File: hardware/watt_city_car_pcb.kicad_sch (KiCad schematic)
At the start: 0 parts

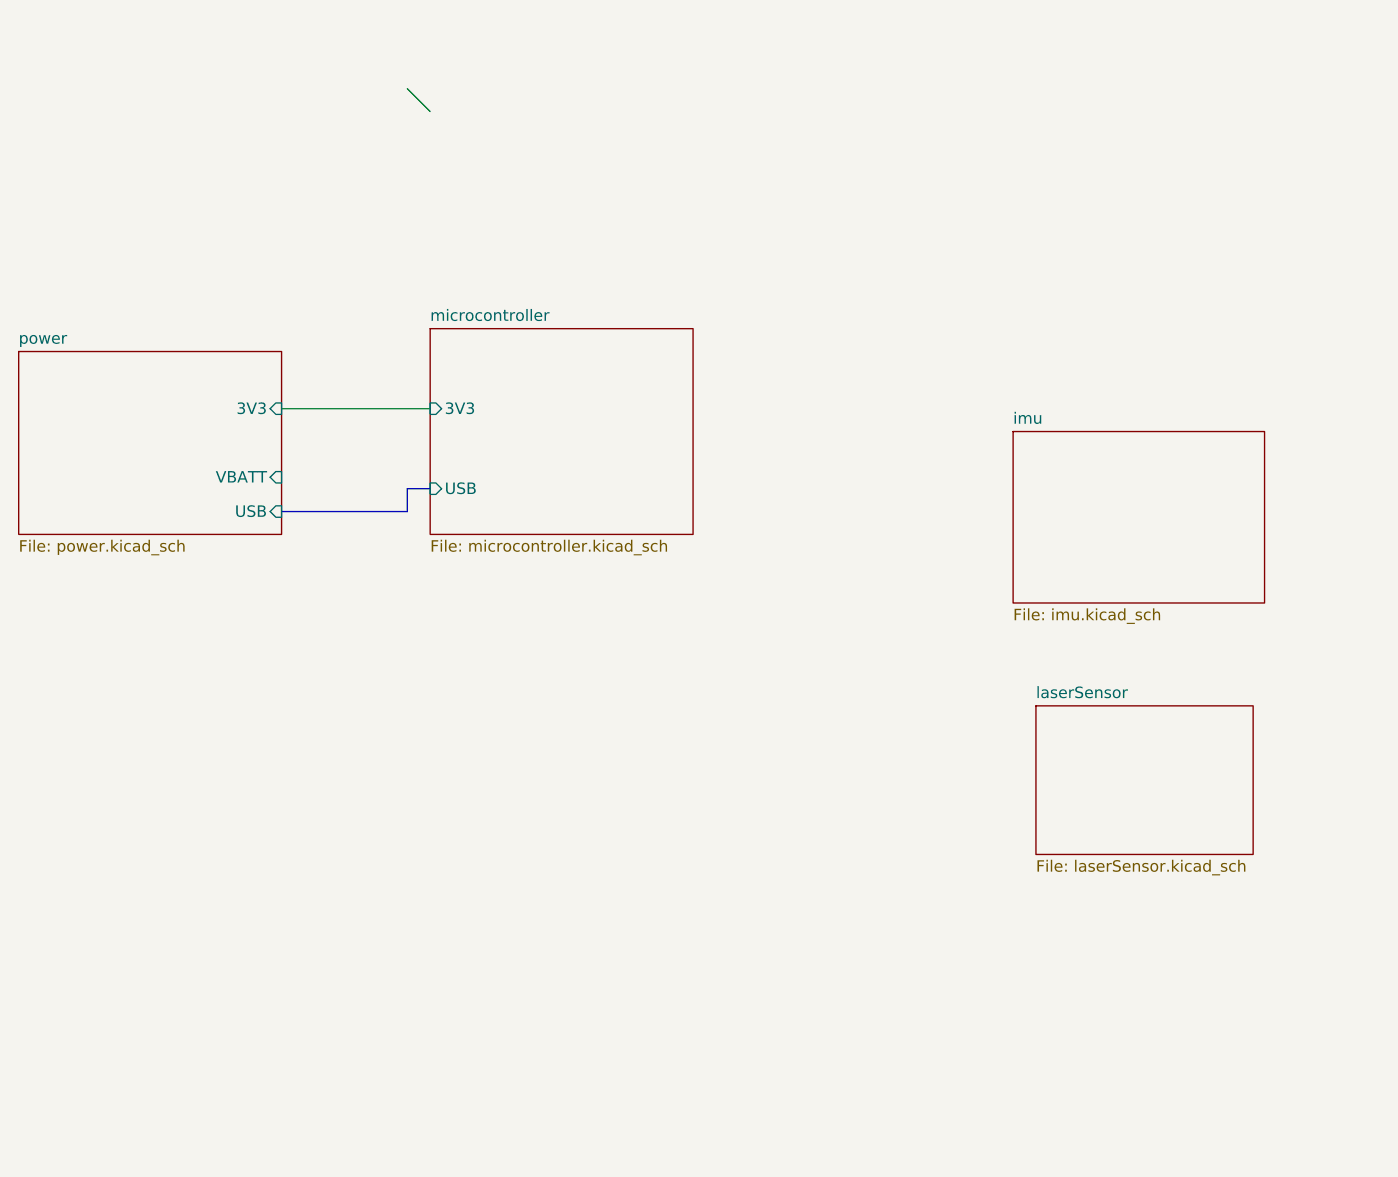
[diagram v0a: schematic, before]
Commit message: updated pcb
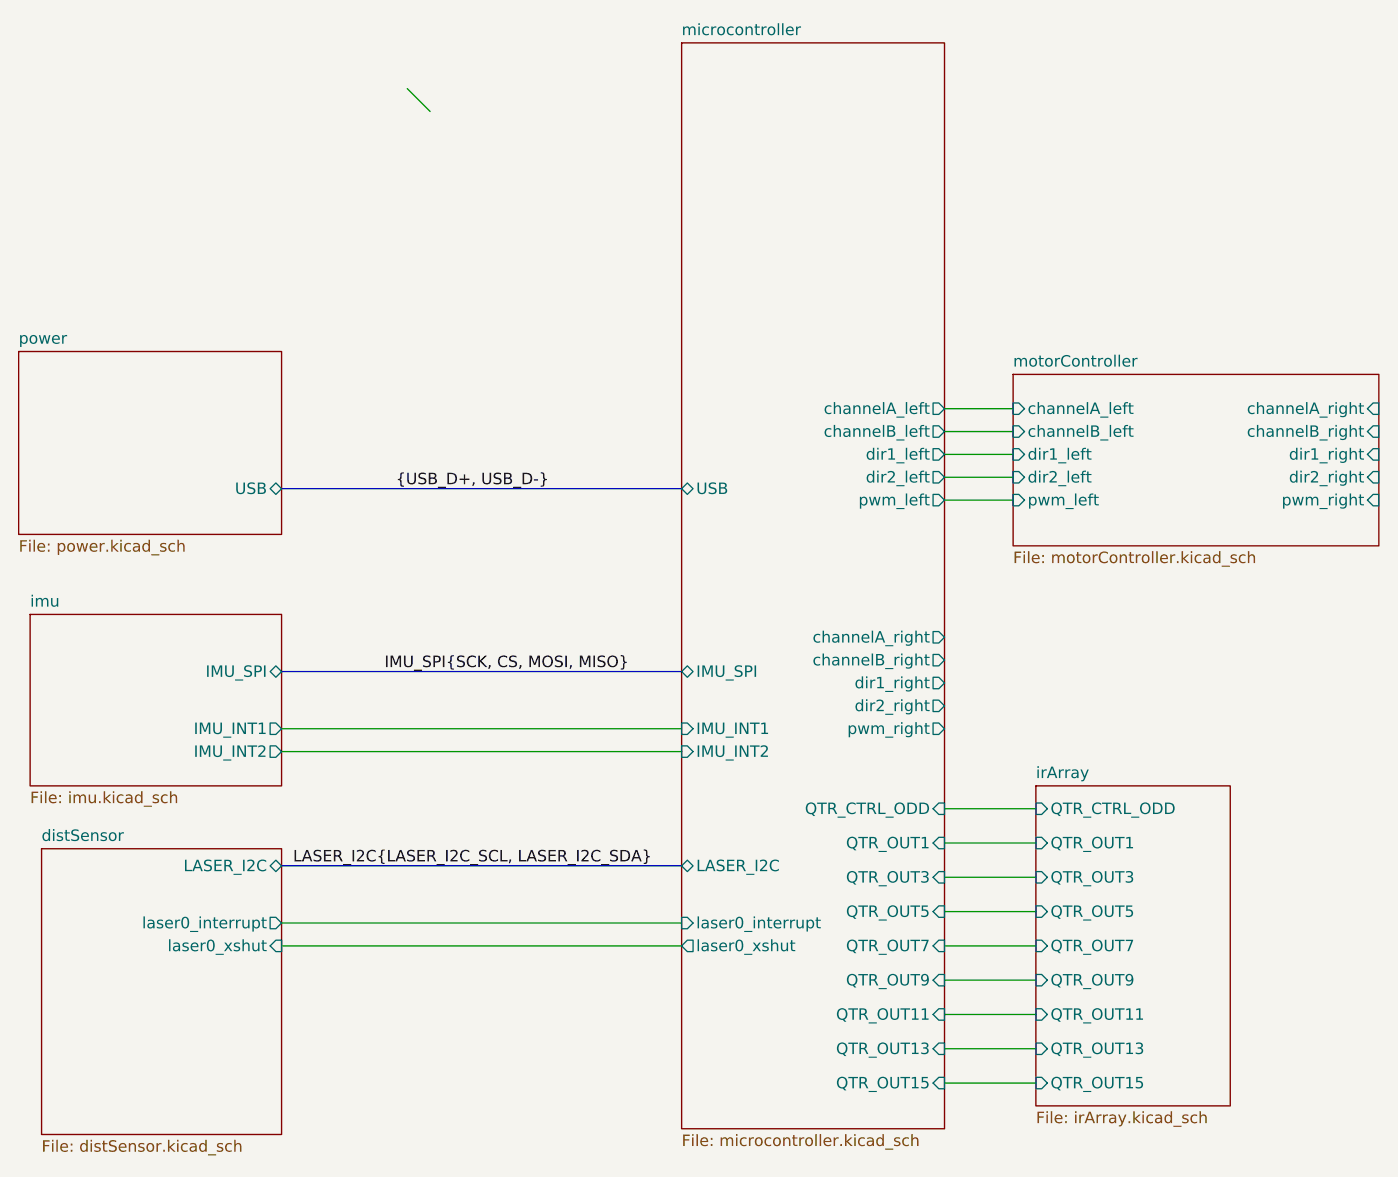
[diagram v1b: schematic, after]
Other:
- removed sheet laserSensor
- added sheet distSensor (distSensor.kicad_sch)
- added sheet irArray (irArray.kicad_sch)
- added sheet motorController (motorController.kicad_sch)
- sheet imu ports: added IMU_INT1, IMU_INT2, IMU_SPI; removed none
- sheet microcontroller ports: added IMU_INT1, IMU_INT2, IMU_SPI, LASER_I2C, QTR_CTRL_ODD, QTR_OUT1, QTR_OUT11, QTR_OUT13, QTR_OUT15, QTR_OUT3, QTR_OUT5, QTR_OUT7, QTR_OUT9, channelA_left, channelA_right, channelB_left, channelB_right, dir1_left, dir1_right, dir2_left, dir2_right, laser0_interrupt, laser0_xshut, pwm_left, pwm_right; removed 3V3
- sheet power ports: added none; removed 3V3, VBATT
